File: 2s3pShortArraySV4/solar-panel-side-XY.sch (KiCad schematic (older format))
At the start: 13 parts, among them J1 2053380005-CONNECTOR, U1 APDS9960_Breakout, U2 DRV2605L_Breakout, U3 MCP9808_Breakout

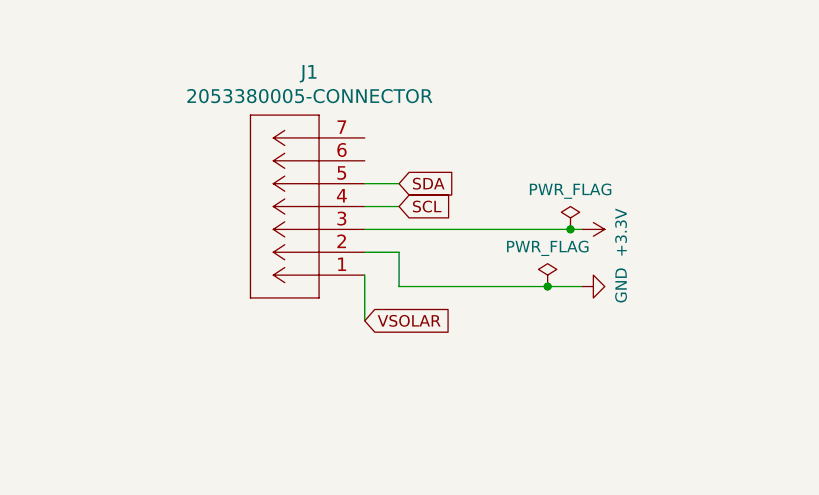
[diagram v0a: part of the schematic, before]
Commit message: Add files via upload
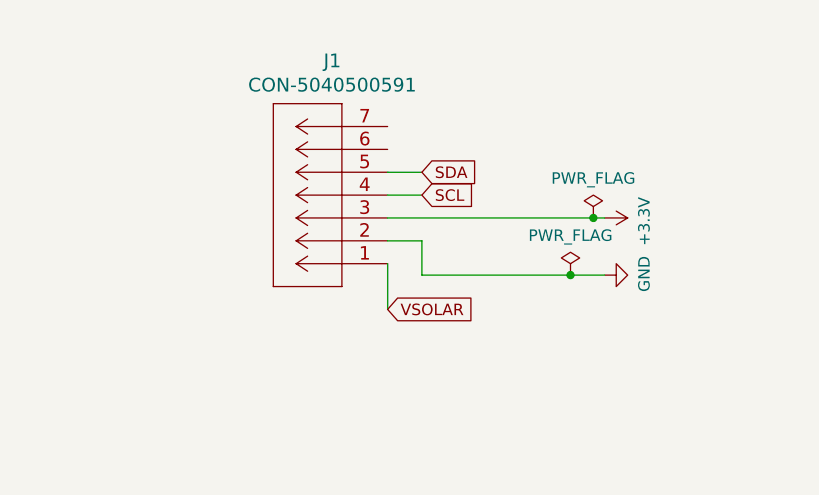
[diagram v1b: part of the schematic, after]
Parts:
- removed J1: 2053380005-CONNECTOR, SolarPanelBoards:CON_2053380005, symbol ExtraComponents:2053380005-CONNECTOR
- added J1: CON-5040500591, SolarPanelBoards:CON_5040500591, symbol ExtraComponents:CON-5040500591
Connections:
- net +3V3: now also J1.3
- net GND: now also J1.2
- net SCL: now also J1.4
- net SDA: now also J1.5
- net VSOLAR: now also J1.1
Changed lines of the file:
@@
 	1    0    0    -1
 $EndComp
-Text GLabel 6850 2300 2    50   Input ~ 0
+Text GLabel 6950 2250 2    50   Input ~ 0
 VSOLAR
 Wire Wire Line
-	6850 2300 6850 2100
+	6950 2250 6950 2050
 $Comp
 L power:GND #PWR0102
 U 1 1 61F725E3
-P 7800 2150
-F 0 "#PWR0102" H 7800 1900 50  0001 C CNN
-F 1 "GND" H 7805 1977 50  0000 C CNN
-F 2 "" H 7800 2150 50  0001 C CNN
-F 3 "" H 7800 2150 50  0001 C CNN
-	1    7800 2150
+P 7900 2100
+F 0 "#PWR0102" H 7900 1850 50  0001 C CNN
+F 1 "GND" H 7905 1927 50  0000 C CNN
+F 2 "" H 7900 2100 50  0001 C CNN
+F 3 "" H 7900 2100 50  0001 C CNN
+	1    7900 2100
 	0    -1   -1   0
 $EndComp
 Wire Wire Line
-	6850 2000 7000 2000
-Wire Wire Line
-	7000 2000 7000 2150
-Wire Wire Line
-	7650 2150 7800 2150
-Connection ~ 7650 2150
+	6950 1950 7100 1950
+Wire Wire Line
+	7100 1950 7100 2100
+Wire Wire Line
+	7750 2100 7900 2100
+Connection ~ 7750 2100
 $Comp
 L power:PWR_FLAG #FLG0104
 U 1 1 61F725D9
-P 7650 2150
-F 0 "#FLG0104" H 7650 2225 50  0001 C CNN
-F 1 "PWR_FLAG" H 7650 2323 50  0000 C CNN
-F 2 "" H 7650 2150 50  0001 C CNN
-F 3 "~" H 7650 2150 50  0001 C CNN
-	1    7650 2150
+P 7750 2100
+F 0 "#FLG0104" H 7750 2175 50  0001 C CNN
+F 1 "PWR_FLAG" H 7750 2273 50  0000 C CNN
+F 2 "" H 7750 2100 50  0001 C CNN
+F 3 "~" H 7750 2100 50  0001 C CNN
+	1    7750 2100
 	1    0    0    -1
 $EndComp
@@
 L power:+3.3V #PWR0111
 U 1 1 61495556
-P 7800 1900
-F 0 "#PWR0111" H 7800 1750 50  0001 C CNN
-F 1 "+3.3V" H 7815 2073 50  0000 C CNN
-F 2 "" H 7800 1900 50  0001 C CNN
-F 3 "" H 7800 1900 50  0001 C CNN
-	1    7800 1900
+P 7900 1850
+F 0 "#PWR0111" H 7900 1700 50  0001 C CNN
+F 1 "+3.3V" H 7915 2023 50  0000 C CNN
+F 2 "" H 7900 1850 50  0001 C CNN
+F 3 "" H 7900 1850 50  0001 C CNN
+	1    7900 1850
 	0    1    1    0
 $EndComp
-Text GLabel 7000 1800 2    50   Input ~ 0
+Text GLabel 7100 1750 2    50   Input ~ 0
 SCL
 $Comp
 L power:PWR_FLAG #FLG0101
 U 1 1 614A3F8B
-P 7750 1900
-F 0 "#FLG0101" H 7750 1975 50  0001 C CNN
-F 1 "PWR_FLAG" H 7750 2073 50  0000 C CNN
-F 2 "" H 7750 1900 50  0001 C CNN
-F 3 "~" H 7750 1900 50  0001 C CNN
-	1    7750 1900
-	1    0    0    -1
-$EndComp
-Connection ~ 7750 1900
-Wire Wire Line
-	7750 1900 7800 1900
-Wire Wire Line
-	7000 2150 7650 2150
-Wire Wire Line
-	6850 1900 7750 1900
-Text GLabel 7000 1700 2    50   Input ~ 0
-SDA
-Wire Wire Line
-	6850 1800 7000 1800
-Wire Wire Line
-	6850 1700 7000 1700
+P 7850 1850
+F 0 "#FLG0101" H 7850 1925 50  0001 C CNN
+F 1 "PWR_FLAG" H 7850 2023 50  0000 C CNN
+F 2 "" H 7850 1850 50  0001 C CNN
+F 3 "~" H 7850 1850 50  0001 C CNN
+	1    7850 1850
+	1    0    0    -1
+$EndComp
+Connection ~ 7850 1850
+Wire Wire Line
+	7850 1850 7900 1850
+Wire Wire Line
+	7100 2100 7750 2100
+Wire Wire Line
+	6950 1850 7850 1850
+Text GLabel 7100 1650 2    50   Input ~ 0
+SDA
+Wire Wire Line
+	6950 1750 7100 1750
+Wire Wire Line
+	6950 1650 7100 1650
 $Comp
 L power:+3.3V #PWR0101
@@
 	3300 3650 3300 3550
 $Comp
-L ExtraComponents:2053380005-CONNECTOR J1
-U 1 1 628744D7
-P 6850 2100
-F 0 "J1" H 7092 1213 60  0000 C CNN
-F 1 "2053380005-CONNECTOR" H 7092 1319 60  0000 C CNN
-F 2 "SolarPanelBoards:CON_2053380005" H 7250 1740 60  0001 C CNN
-F 3 "" H 6850 2100 60  0000 C CNN
-	1    6850 2100
+L ExtraComponents:CON-5040500591 J1
+U 1 1 62783659
+P 6950 2050
+F 0 "J1" H 7192 1163 60  0000 C CNN
+F 1 "CON-5040500591" H 7192 1269 60  0000 C CNN
+F 2 "SolarPanelBoards:CON_5040500591" H 7350 1690 60  0001 C CNN
+F 3 "" H 6950 2050 60  0000 C CNN
+	1    6950 2050
 	-1   0    0    1
 $EndComp
